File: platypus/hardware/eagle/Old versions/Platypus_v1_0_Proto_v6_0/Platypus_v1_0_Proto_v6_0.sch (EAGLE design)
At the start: 27 parts, among them IC1 MPU-9250, J1 EDISON_CONNECTOR_FULLMOUNTING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, U2 TXB0108, U3 MAX17043, X3 Power TP, X4 I2C TP, X5 Display TP

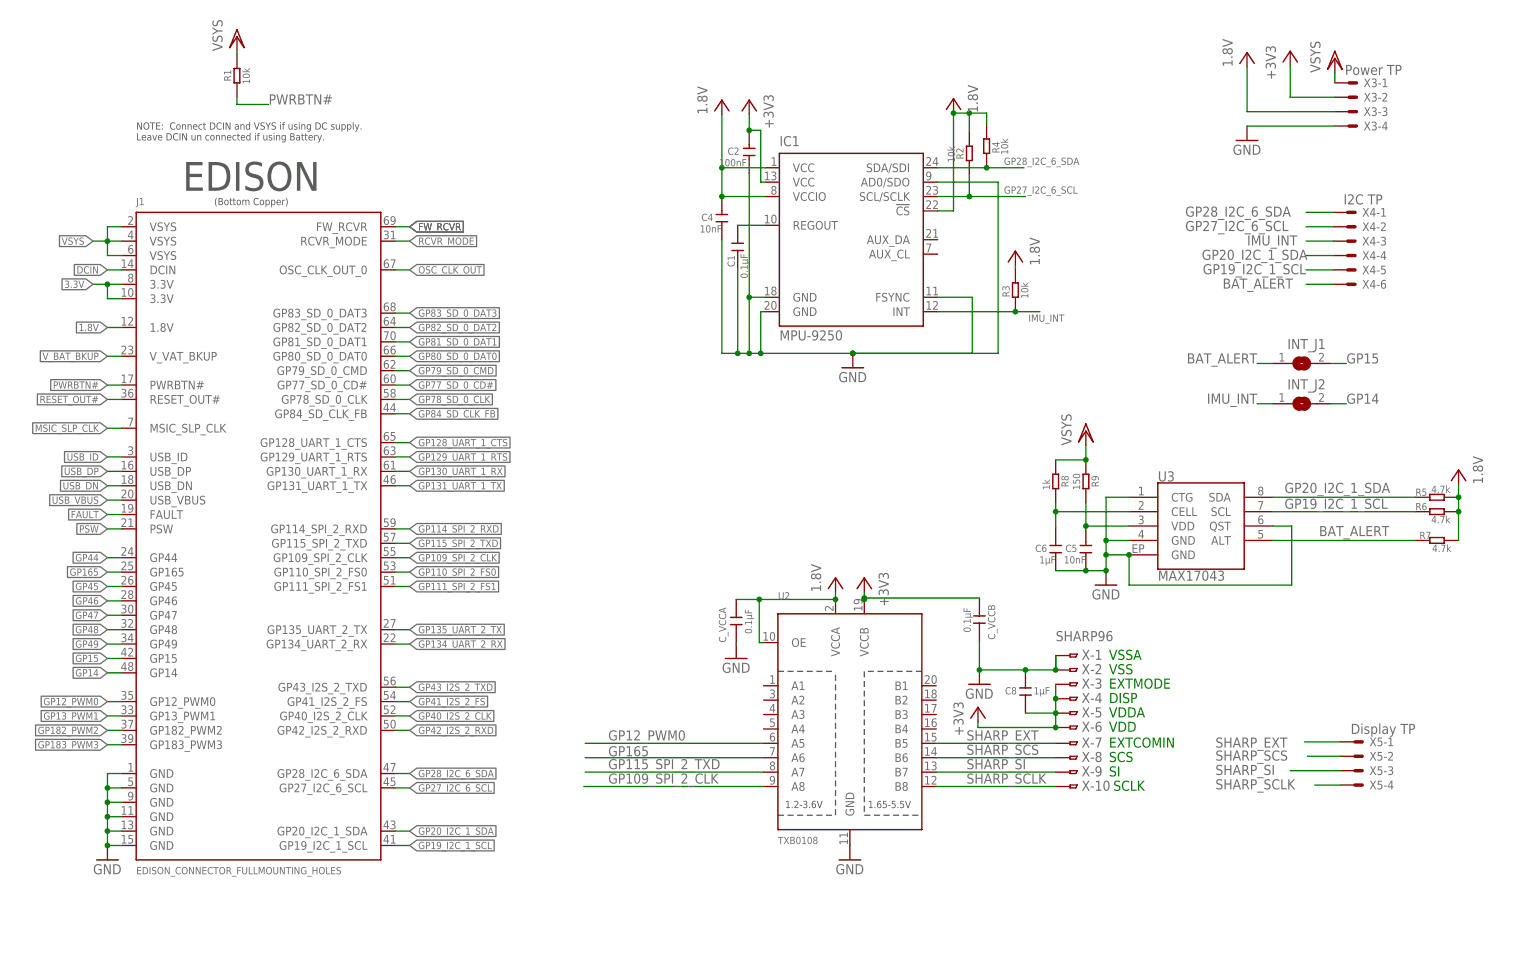
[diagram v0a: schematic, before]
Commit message: updated platypus hardware folder
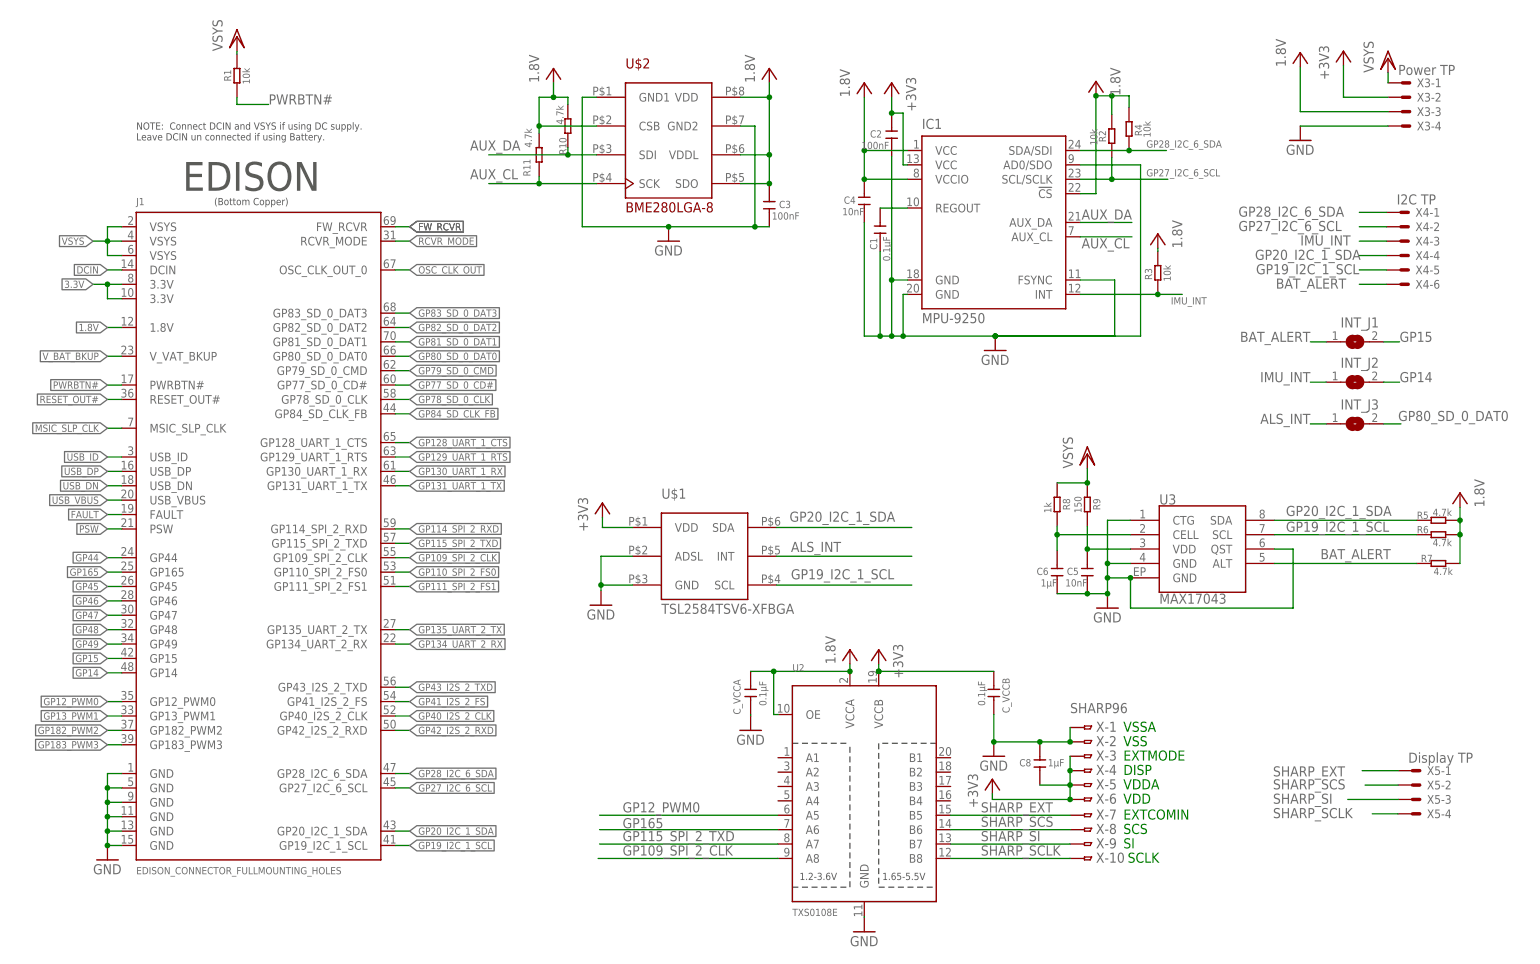
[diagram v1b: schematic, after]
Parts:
- added C3: 100nF, Discrete:C-0603
- added INT_J3: (no value), jumper:SJ
- added R10, R11: 4.7k, Discrete:R-0603
- added U$1: TSL2584TSV6-XFBGA, TSL2584TSV:TSL2584TSV6-XFBGA
- added U$2: BME280LGA-8, BME280:BME280LGA-8
- U2: value TXB0108 -> TXS0108E
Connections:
- new net ALS_INT: INT_J3.1, U$1.INT
- new net AUX_CL: IC1.AUX_CL, R11.1, U$2.SCK
- new net AUX_DA: IC1.AUX_DA, R10.1, U$2.SDI
- net 1.8V: now also C3.2, R10.2, R11.2, U$2.CSB, U$2.SDO, U$2.VDD, U$2.VDDL
- net 3.3V: now also U$1.VDD
- net GND: now also C3.1, U$1.ADSL, U$1.GND, U$2.GND1, U$2.GND2
- net GP19_I2C_1_SCL: now also U$1.SCL
- net GP20_I2C_1_SDA: now also U$1.SDA
- net GP80_SD_0_DAT0: now also INT_J3.2
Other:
- moved on the sheet: C1, C2, C4, C5, C6, C8, C_VCCA, C_VCCB, IC1, INT_J1, INT_J2, R2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
